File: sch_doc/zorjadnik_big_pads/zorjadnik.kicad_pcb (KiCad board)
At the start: 2 copper layers, 65 parts, among them J1 OUT1, J10 output GND, J11 power supply GND, J12 spare port, J2 OUT2, J3 Vsb, J4 GND, J5 display module, J6 firmware, J7 cooling fan, J8 driver, J9 power supply Vout, Q1 BCR512, Q2 BCR108, Q3 BCR108, U1 AP1117-33, U2 STM32F030F4Px, U3 74HC595, U4 74HC595

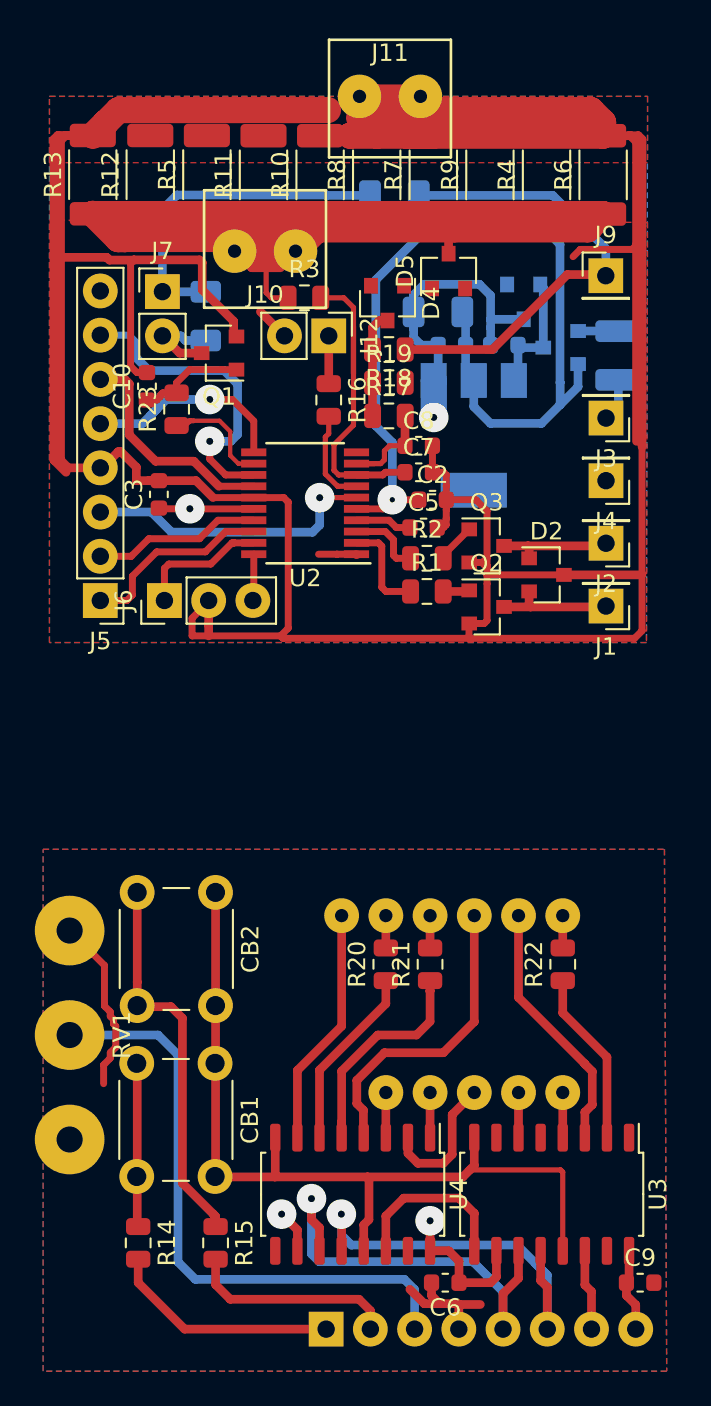
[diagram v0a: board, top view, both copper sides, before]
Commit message: поаккуратней схема
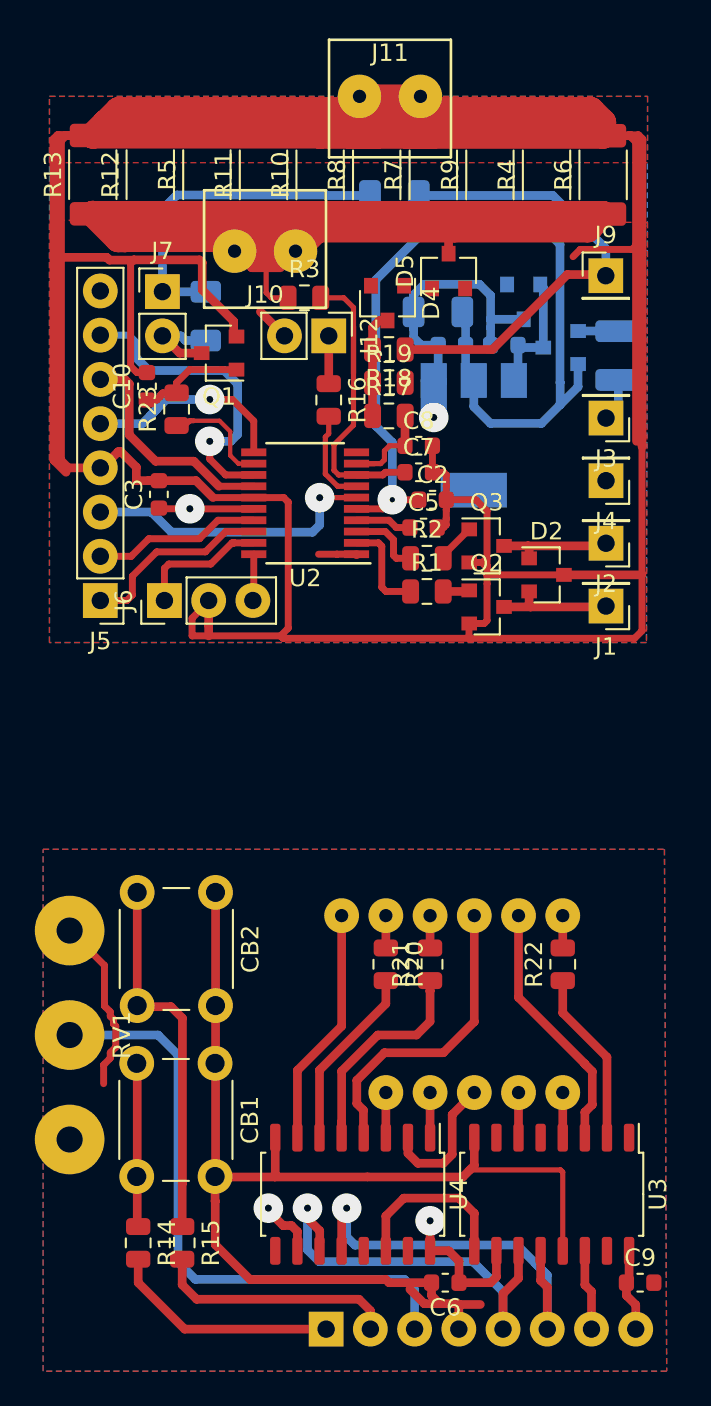
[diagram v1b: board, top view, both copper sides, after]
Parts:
- moved R15 1.92 mm to (30.8, 87.0)
- turned R20 to 270 degrees
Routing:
- net GND: track 342.8 -> 374.0 mm
- net Net-(J8-Pad2): track 12.0 -> 14.0 mm
- net Net-(J8-Pad6): track 24.5 -> 25.5 mm
- net +3V3: track 73.4 -> 74.3 mm
- net Net-(J8-Pad5): track 24.9 -> 24.0 mm
- net Net-(CB2-Pad2): track 22.1 -> 21.3 mm
